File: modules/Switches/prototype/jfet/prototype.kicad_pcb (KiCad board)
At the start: 6 copper layers, 40.6 x 78.7 mm, 15 parts, among them J1 Conn_01x09, Q1 J109/J112, Q2 J109/J112, Q3 2N3906, SW1 SW_Push, U1 TL072

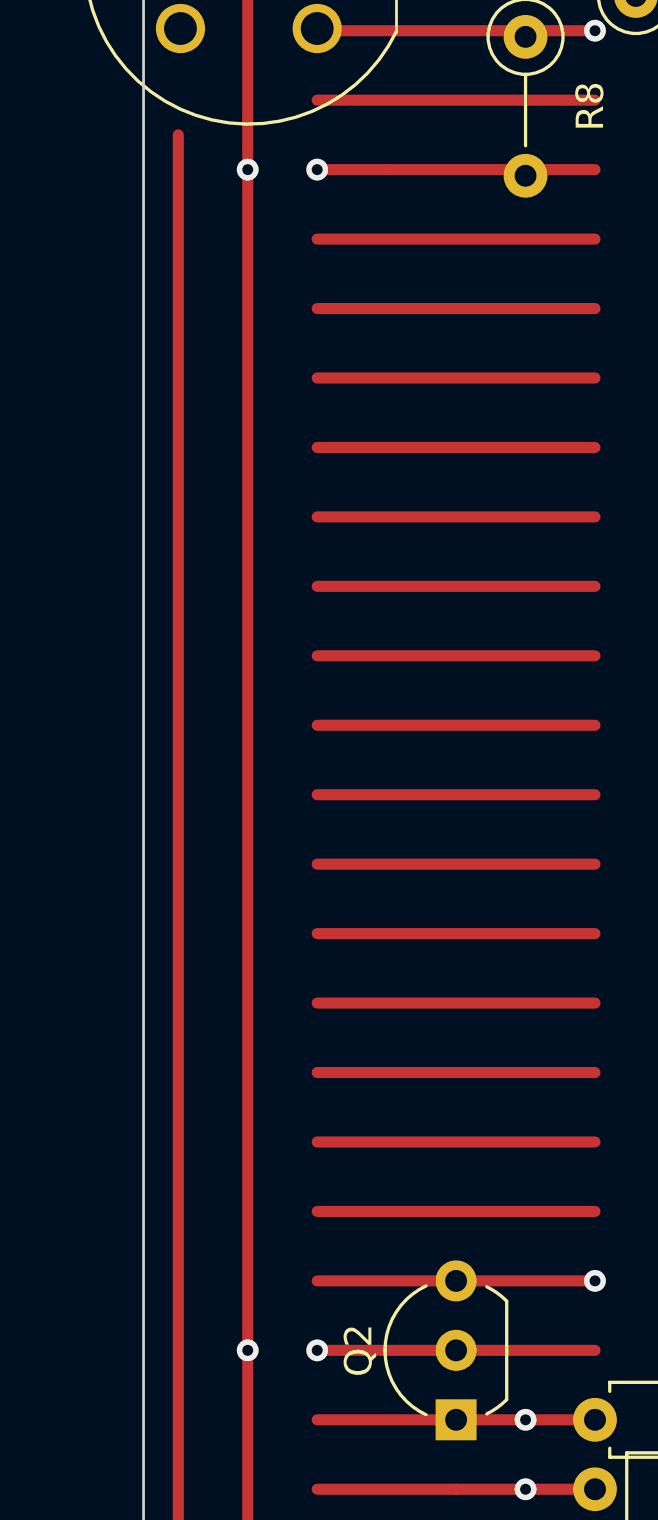
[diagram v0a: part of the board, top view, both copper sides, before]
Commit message: Switches module - prototype wip
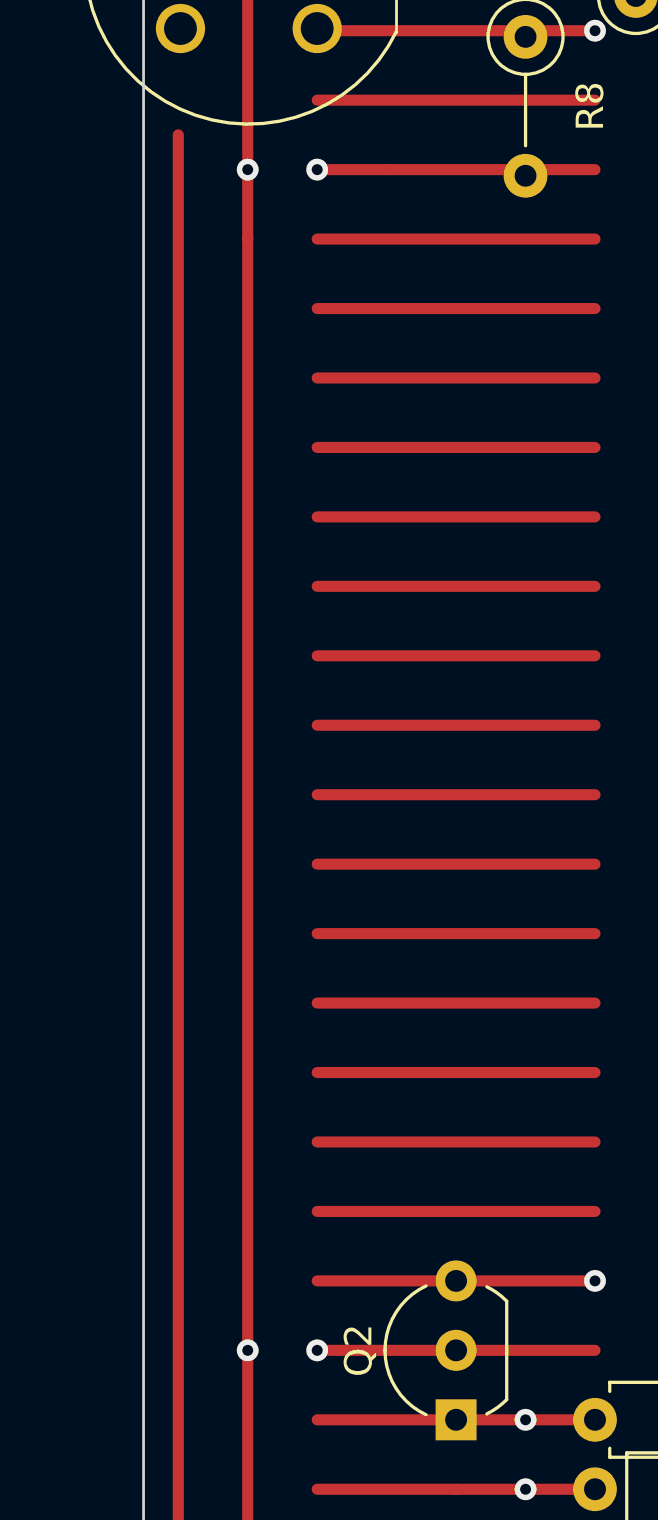
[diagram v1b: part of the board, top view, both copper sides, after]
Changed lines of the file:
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@@
   (segment (start 119.38 95.25) (end 119.38 95.25) (width 0.4064) (layer "F.Cu") (net 2))
   (segment (start 86.36 95.25) (end 86.36 95.25) (width 0.4064) (layer "F.Cu") (net 2))
-  (segment (start 86.36 35.56) (end 86.36 78.74) (width 0.4064) (layer "F.Cu") (net 2))
+  (segment (start 86.36 35.56) (end 86.36 38.1) (width 0.4064) (layer "F.Cu") (net 2))
   (segment (start 119.38 78.74) (end 119.38 95.25) (width 0.4064) (layer "F.Cu") (net 2))
   (segment (start 86.36 78.74) (end 86.36 95.25) (width 0.4064) (layer "F.Cu") (net 2))
   (segment (start 99.06 35.56) (end 91.44 35.56) (width 0.4064) (layer "F.Cu") (net 2))
+  (segment (start 86.36 38.1) (end 86.36 78.74) (width 0.4064) (layer "F.Cu") (net 2))
   (segment (start 119.38 30.48) (end 119.38 78.74) (width 0.4064) (layer "F.Cu") (net 2))
   (segment (start 91.44 35.56) (end 88.9 35.56) (width 0.4064) (layer "F.Cu") (net 2))
   (via (at 119.38 95.25) (size 0.8) (drill 0.4) (layers "F.Cu" "B.Cu") (net 2))
   (via (at 86.36 78.74) (size 0.8) (drill 0.4) (layers "F.Cu" "B.Cu") (net 2))
-  (via (at 86.36 35.56) (size 0.8) (drill 0.4) (layers "F.Cu" "B.Cu") (net 2))
   (via (at 88.9 78.74) (size 0.8) (drill 0.4) (layers "F.Cu" "B.Cu") (net 2))
   (via (at 119.38 78.74) (size 0.8) (drill 0.4) (layers "F.Cu" "B.Cu") (net 2))
@@
   (via (at 86.36 95.25) (size 0.8) (drill 0.4) (layers "F.Cu" "B.Cu") (net 2))
   (via (at 116.84 78.74) (size 0.8) (drill 0.4) (layers "F.Cu" "B.Cu") (net 2))
+  (via (at 86.36 35.56) (size 0.8) (drill 0.4) (layers "F.Cu" "B.Cu") (net 2))
   (segment (start 88.9 35.56) (end 86.36 35.56) (width 0.4064) (layer "In1.Cu") (net 2))
   (segment (start 88.9 78.74) (end 86.36 78.74) (width 0.4064) (layer "In1.Cu") (net 2))

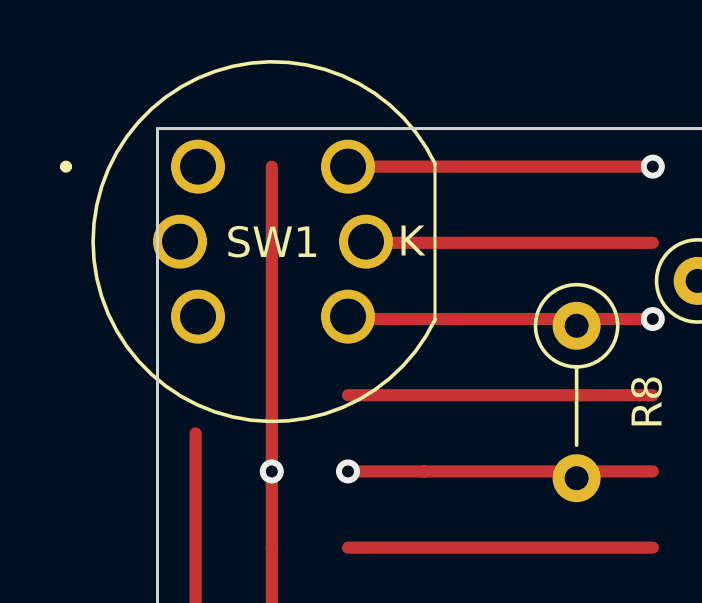
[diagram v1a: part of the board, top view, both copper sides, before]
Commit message: Switches module - prototype - wip
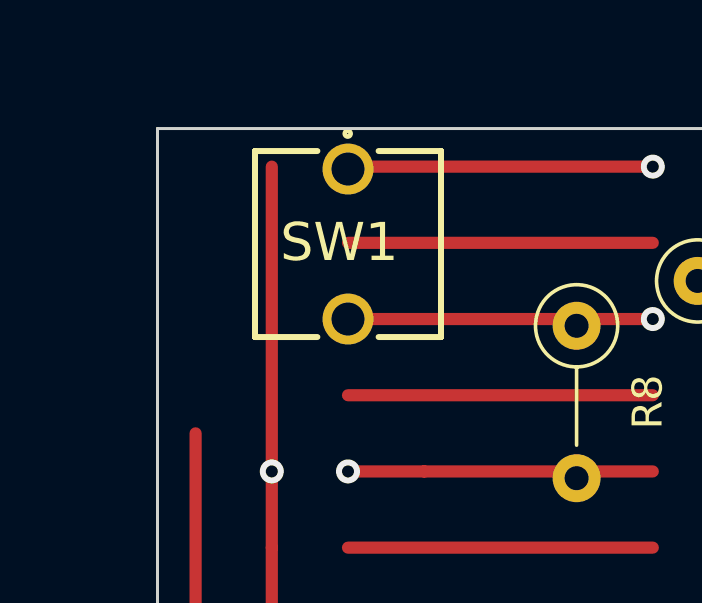
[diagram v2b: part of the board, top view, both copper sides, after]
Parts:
- SW1: footprint -lmp-synth:SW_Push_LED_C&K_D6R -> -lmp-misc:SW_PUSH_6mm_2
- moved SW1 5.63 mm to (88.9, 28.0)
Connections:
- SW1 pad 1: unconnected-(SW1-Pad1) -> +5V
- SW1 pad 2: +5V -> Net-(R7-Pad1)
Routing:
- net unconnected-(SW1-K-Pad6): track 10.2 -> 0.00 mm
- net (no net): track 335.3 -> 345.4 mm
